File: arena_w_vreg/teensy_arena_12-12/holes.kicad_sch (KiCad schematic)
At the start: 4 parts

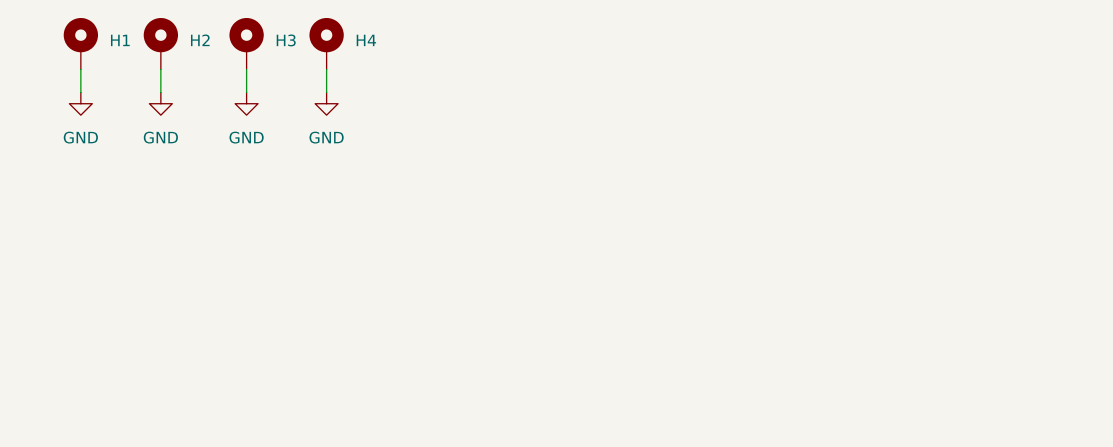
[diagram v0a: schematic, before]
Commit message: Wored on teensy arena.
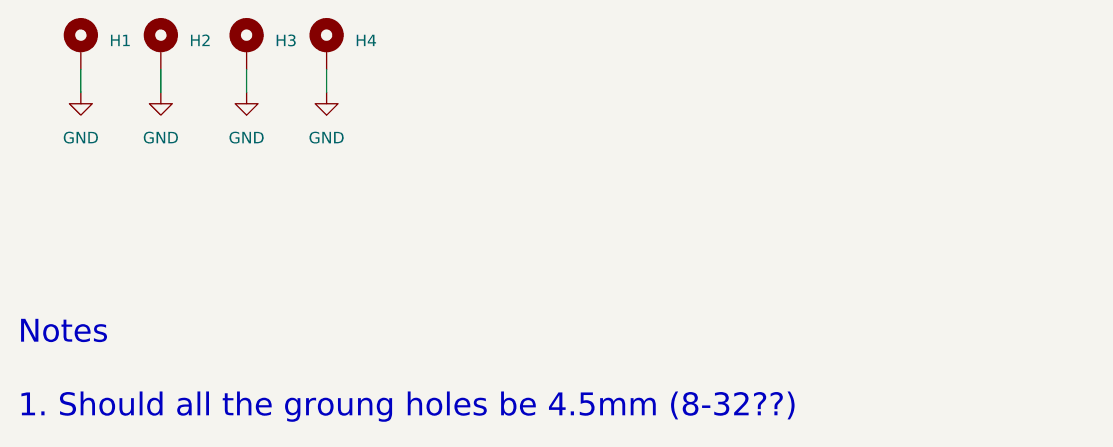
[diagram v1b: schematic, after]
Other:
- note added: "Notes 1. Should all the groung holes be 4.5mm (8-32??)"
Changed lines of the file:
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@@
     (stroke (width 0) (type default))
+  )
+  (text "Notes\n\n1. Should all the groung holes be 4.5mm (8-32??)\n"
+    (at 34.29 71.628 0)
+    (effects (font (size 2.54 2.54)) (justify left bottom))
   )
   (symbol (lib_id "power:GND") (at 68.58 35.179 0) (mirror y) (unit 1)
